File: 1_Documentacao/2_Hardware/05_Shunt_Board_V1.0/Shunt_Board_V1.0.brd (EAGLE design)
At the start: 88 x 17.5 mm, 17 parts

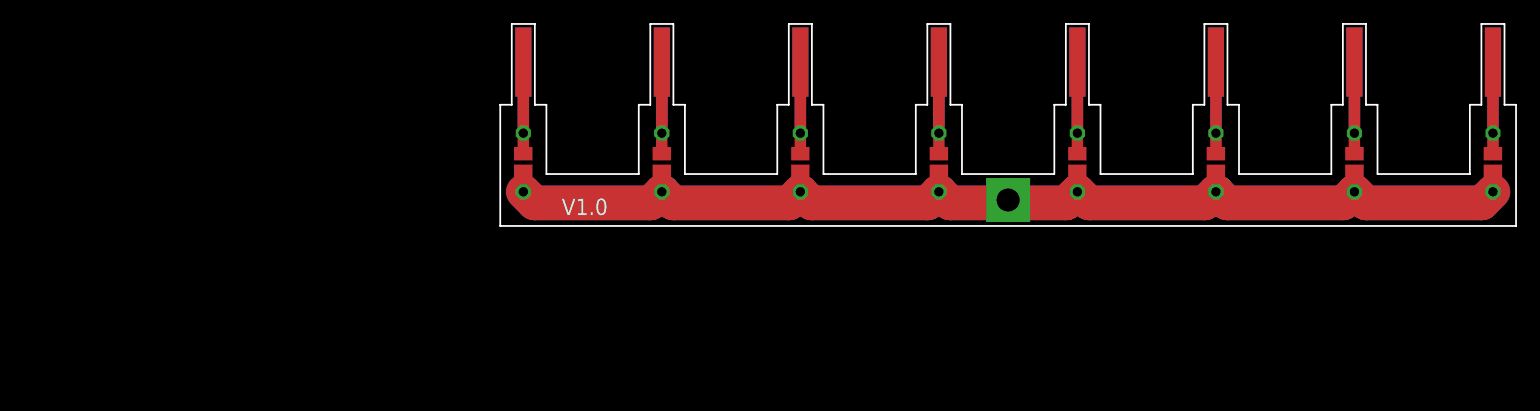
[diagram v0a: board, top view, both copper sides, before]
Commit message: Update Hardware Files
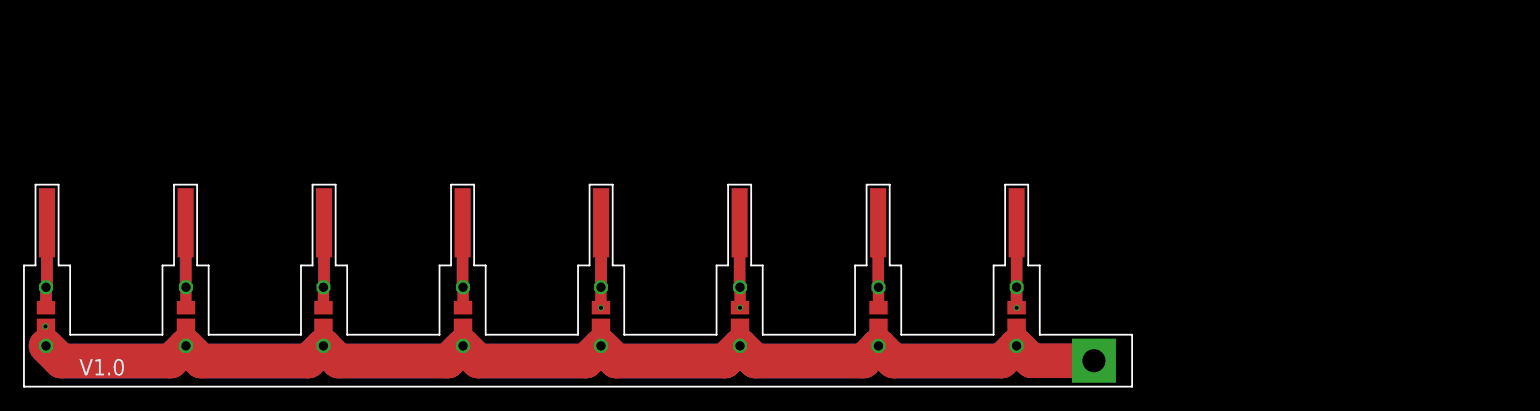
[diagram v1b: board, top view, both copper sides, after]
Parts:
- removed U$28: SHUNT2, Shunt2:SHUNT2
- added U$1: SHUNT, Shunt_V1.0:SHUNT
- moved R11 43.5 mm to (-108.0, 6.35)
- moved SJ20 43.5 mm to (-108.0, 6.35)
- moved R19 43.4 mm to (-83.9, 6.35)
- moved SJ22 43.4 mm to (-83.9, 6.35)
- moved SJ10 43.4 mm to (-59.9, 6.35)
- moved R21 43.4 mm to (-59.9, 6.35)
- moved R24 43.4 mm to (-23.9, 6.35)
- moved SJ19 43.4 mm to (-23.9, 6.35)
- moved R23 43.3 mm to (-35.8, 6.35)
- moved SJ17 43.3 mm to (-35.8, 6.35)
- moved R18 43.3 mm to (-95.8, 6.35)
- moved SJ21 43.3 mm to (-95.8, 6.35)
- moved R22 43.3 mm to (-47.8, 6.35)
- moved SJ24 43.3 mm to (-47.8, 6.35)
- moved R20 43.3 mm to (-71.8, 6.35), flipped to the bottom
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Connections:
- removed net N$94: R21.2, SJ10.2, U$28.P$14, U$28.P$5
- removed net N$95: R22.2, SJ24.2, U$28.P$15, U$28.P$6
- removed net N$98: R11.1, R18.1, R19.1, R20.1, R21.1, R22.1, R23.1, R24.1, SJ10.1, SJ17.1, SJ19.1, SJ20.1, SJ21.1, SJ22.1, SJ23.1, SJ24.1, U$28.P$18
- new net N$1: R11.1, R18.1, R19.1, R20.1, R21.1, R22.1, R23.1, R24.1, SJ10.1, SJ17.1, SJ19.1, SJ20.1, SJ21.1, SJ22.1, SJ23.1, SJ24.1, U$1.P$9
- new net N$2: R21.2, SJ10.2, U$1.P$5
- new net N$4: R22.2, SJ24.2, U$1.P$6
- net N$91: now also U$1.P$2; no longer U$28.P$11, U$28.P$2
- net N$92: now also U$1.P$3; no longer U$28.P$12, U$28.P$3
- net N$93: now also U$1.P$4; no longer U$28.P$13, U$28.P$4
- net N$96: now also U$1.P$7; no longer U$28.P$16, U$28.P$7
- net N$97: now also U$1.P$8; no longer U$28.P$17, U$28.P$8
- net N$99: now also U$1.P$1; no longer U$28.P$1, U$28.P$10
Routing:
- net N$1: track 0.00 -> 228.0 mm, vias 0 -> 8
- net N$98: track 196.6 -> 0.00 mm
- net N$95: track 14.1 -> 0.00 mm
- net N$94: track 14.1 -> 0.00 mm
- net N$4: track 0.00 -> 13.0 mm, vias 0 -> 1
- net N$2: track 0.00 -> 13.0 mm, vias 0 -> 1
- net N$91: track 14.1 -> 13.0 mm
- net N$93: track 14.1 -> 13.0 mm
- net N$96: track 14.1 -> 13.0 mm
- net N$92: track 14.1 -> 13.0 mm
- net N$99: track 14.1 -> 14.8 mm
- net N$97: track 14.1 -> 14.7 mm, vias 0 -> 1
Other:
- board size 88 x 17.5 mm -> 96 x 17.5 mm
